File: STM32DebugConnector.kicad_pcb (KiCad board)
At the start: 2 copper layers, 20 x 20 mm, 12 parts, among them J1 USB_B_Micro, J2 STM32_Debug, J3 STDC32, SW1 RESET, U1 NJM2884U1

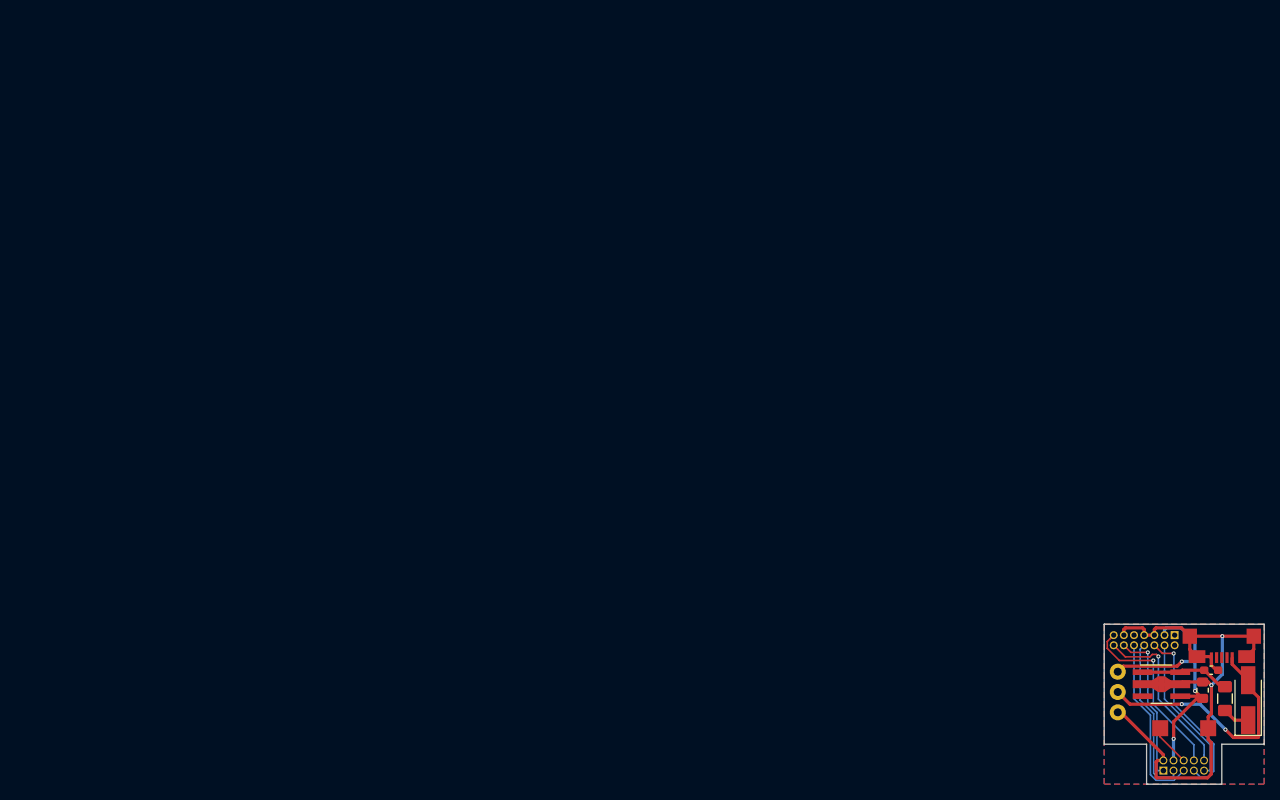
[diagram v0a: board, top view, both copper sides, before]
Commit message: 基板 V2.0
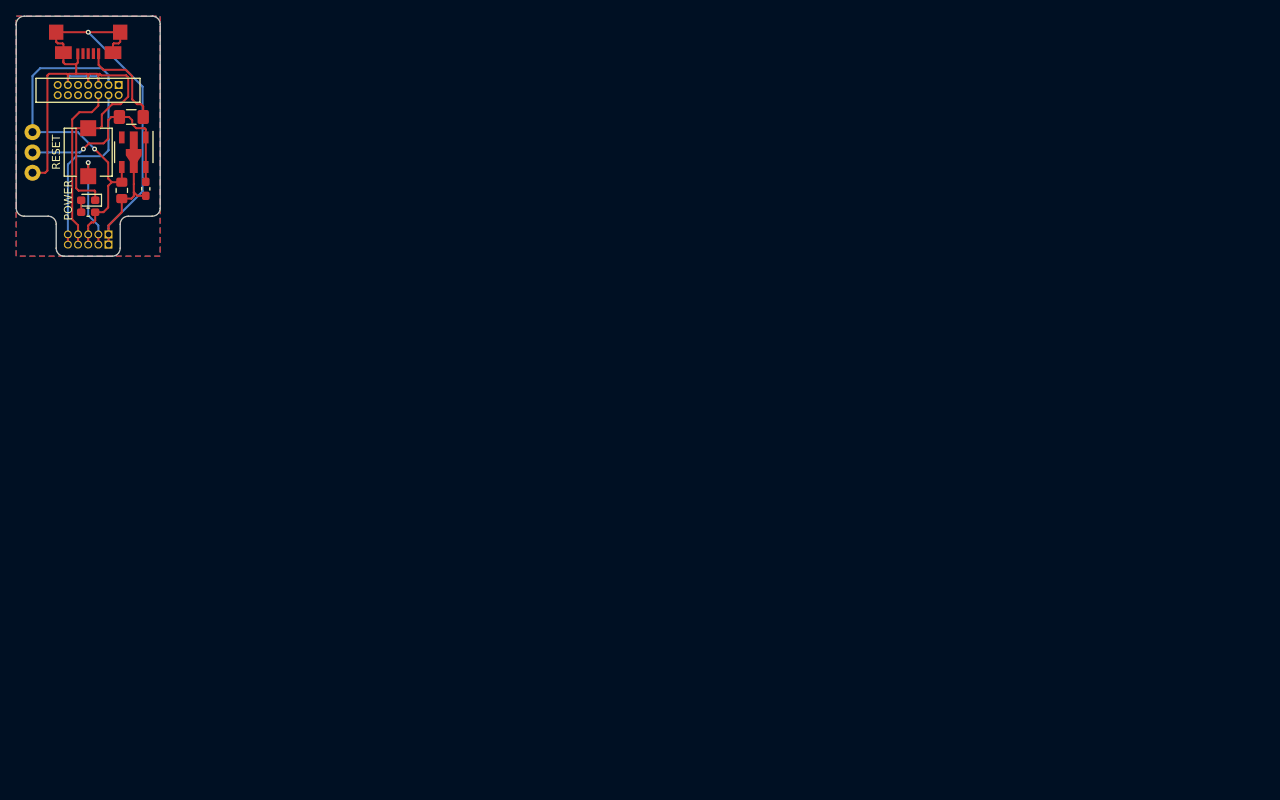
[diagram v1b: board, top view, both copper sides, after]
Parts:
- added J4: STM32_Debug_5pin, STM32DebugConnector:STM32_Debug_5pin, F.Cu at (2.54, 28.6)
- added R1: R, Resistor_SMD:R_0603_1608Metric_Pad1.05x0.95mm_HandSolder, F.Cu at (0.00, 24.5)
- D1: value SS14 -> Power; footprint Diode_SMD:D_SMA_Handsoldering -> LED_SMD:LED_0603_1608Metric_Pad1.05x0.95mm_HandSolder
- J2: value STM32_Debug -> STDC32; footprint Connector_PinSocket_1.27mm:PinSocket_2x05_P1.27mm_Vertical -> Connector_PinHeader_1.27mm:PinHeader_2x07_P1.27mm_Vertical; moved to F.Cu
- J3: value STDC32 -> STM32_Debug_5pin; footprint Connector_PinHeader_1.27mm:PinHeader_2x07_P1.27mm_Vertical -> STM32DebugConnector:STM32_Debug_5pin
- U1: footprint Package_TO_SOT_SMD:SOT-89-5_Handsoldering -> Package_TO_SOT_SMD:SOT-89-5
- moved J1 160.6 mm to (0.00, 2.00)
- moved D1 157.9 mm to (0.00, 23.0), turned to 180 degrees
- moved J2 156.2 mm to (3.81, 8.60)
- moved F1 154.8 mm to (5.39, 12.6), turned to 0 degrees
- moved SW1 154.8 mm to (0.00, 17.0), turned to 90 degrees
- moved TP1 151.5 mm to (-6.96, 17.0)
- moved TP2 151.5 mm to (-6.96, 14.5)
- moved TP3 151.5 mm to (-6.96, 19.6)
- moved C2 148.8 mm to (4.20, 21.8), turned to 270 degrees
- moved C1 146.1 mm to (7.20, 21.6), turned to 270 degrees
- moved U1 144.6 mm to (5.70, 17.0), turned to 270 degrees
- moved J3 142.4 mm to (2.54, 27.3)
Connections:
- C1 pad 1: Net-(C1-Pad1) -> +5V
- D1 pad 1: Net-(D1-Pad1) -> GND
- D1 pad 2: +5V -> Net-(D1-Pad2)
- F1 pad 1: Net-(C1-Pad1) -> +5V
- F1 pad 2: Net-(D1-Pad1) -> Net-(F1-Pad2)
- J1 pad 1: +5V -> Net-(F1-Pad2)
- J2 pad 1: Net-(J2-Pad1) -> (no net)
- J2 pad 10: Net-(J2-Pad10) -> (no net)
- J2 pad 2: GND -> (no net)
- J2 pad 3: Net-(J2-Pad3) -> +3V0
- J2 pad 4: +3V0 -> SWDIO
- J2 pad 5: Net-(J2-Pad5) -> GND
- J2 pad 6: Net-(J2-Pad6) -> SWCLK
- J2 pad 7: Net-(J2-Pad7) -> GND
- J2 pad 8: Net-(J2-Pad8) -> (no net)
- J2 pad 9: Net-(J2-Pad9) -> (no net)
- J3 pad 1: (no net) -> GND
- J3 pad 2: (no net) -> NRST
- J3 pad 4: Net-(J2-Pad9) -> SWCLK
- J3 pad 5: GND -> SWDIO
- SW1 pad 1: Net-(J2-Pad6) -> NRST
- U1 pad 1: Net-(C1-Pad1) -> +5V
- U1 pad 5: Net-(C1-Pad1) -> +5V
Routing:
- net GND: track 74.5 -> 124.4 mm, vias 2 -> 1
- net Net-(J2-Pad8): track 23.0 -> 0.00 mm, vias 1 -> 0
- net Net-(J2-Pad7): track 22.7 -> 0.00 mm, vias 1 -> 0
- net SWDIO: track 0.00 -> 22.7 mm
- net Net-(J2-Pad5): track 22.0 -> 0.00 mm
- net Net-(J2-Pad10): track 21.8 -> 0.00 mm, vias 1 -> 0
- net SWCLK: track 0.00 -> 21.2 mm
- net Net-(J2-Pad3): track 20.3 -> 0.00 mm
- net Net-(J2-Pad1): track 19.4 -> 0.00 mm, vias 1 -> 0
- net Net-(J2-Pad9): track 18.8 -> 0.00 mm
- net NRST: track 0.00 -> 12.5 mm, vias 0 -> 1
- net Net-(F1-Pad2): track 0.00 -> 12.2 mm
- net Net-(C1-Pad1): track 11.2 -> 0.00 mm
- net +3V0: track 35.6 -> 45.1 mm, vias 3 -> 1
- net +5V: track 31.3 -> 24.8 mm, vias 2 -> 1
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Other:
- board size 20 x 20 mm -> 18 x 30 mm
- net class Default: trace_width 0.2032 -> 0.254; via_dia 0.508 -> 0.6096; via_drill 0.254 -> 0.3048
- rule via_min_drill: 0.254 -> 0.3048
- rule via_min_size: 0.508 -> 0.6096
- board text added: "NRST"
- board text added: "POWER"
- board text added: "RESET"
- board text added: "STM32 Debug Connector V2.0"
- board text added: "SWCLK"
- board text added: "SWDIO"
- board text added: "VDD"
